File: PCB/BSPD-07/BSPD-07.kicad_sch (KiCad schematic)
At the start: 55 parts, among them IC1 LM393LVQDRQ1, IC2 LM393LVQDRQ1, IC3 LM393LVQDRQ1, IC4 LDO40LPU50RY, IC5 74LVC1G02GW-Q100H, J1 DTM13-12PA, Q1 RSQ025P03HZGTR, Q2 RJU002N06FRAT106, Q3 RJU002N06FRAT106, U2 TLP175A / COMUS AB38-Q

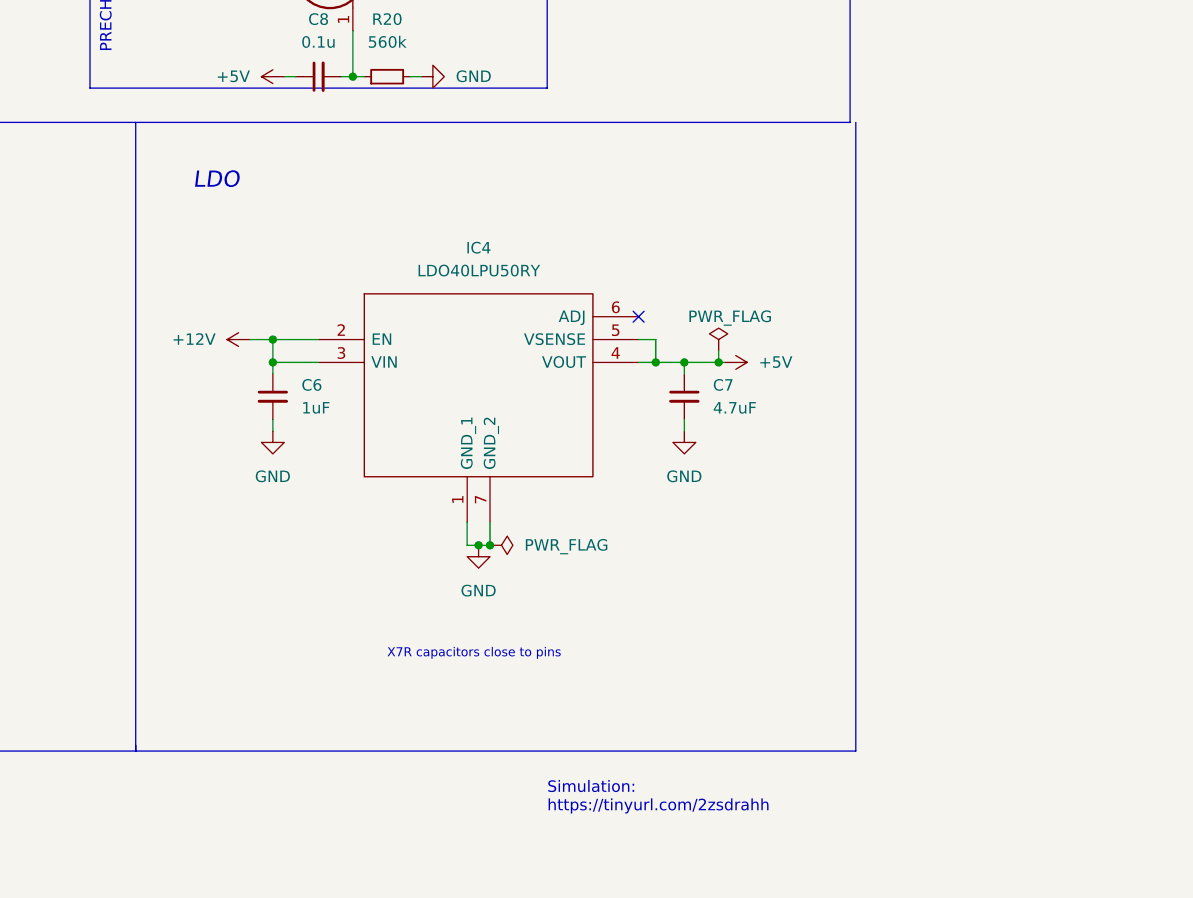
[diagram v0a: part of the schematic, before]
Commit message: Revised layout
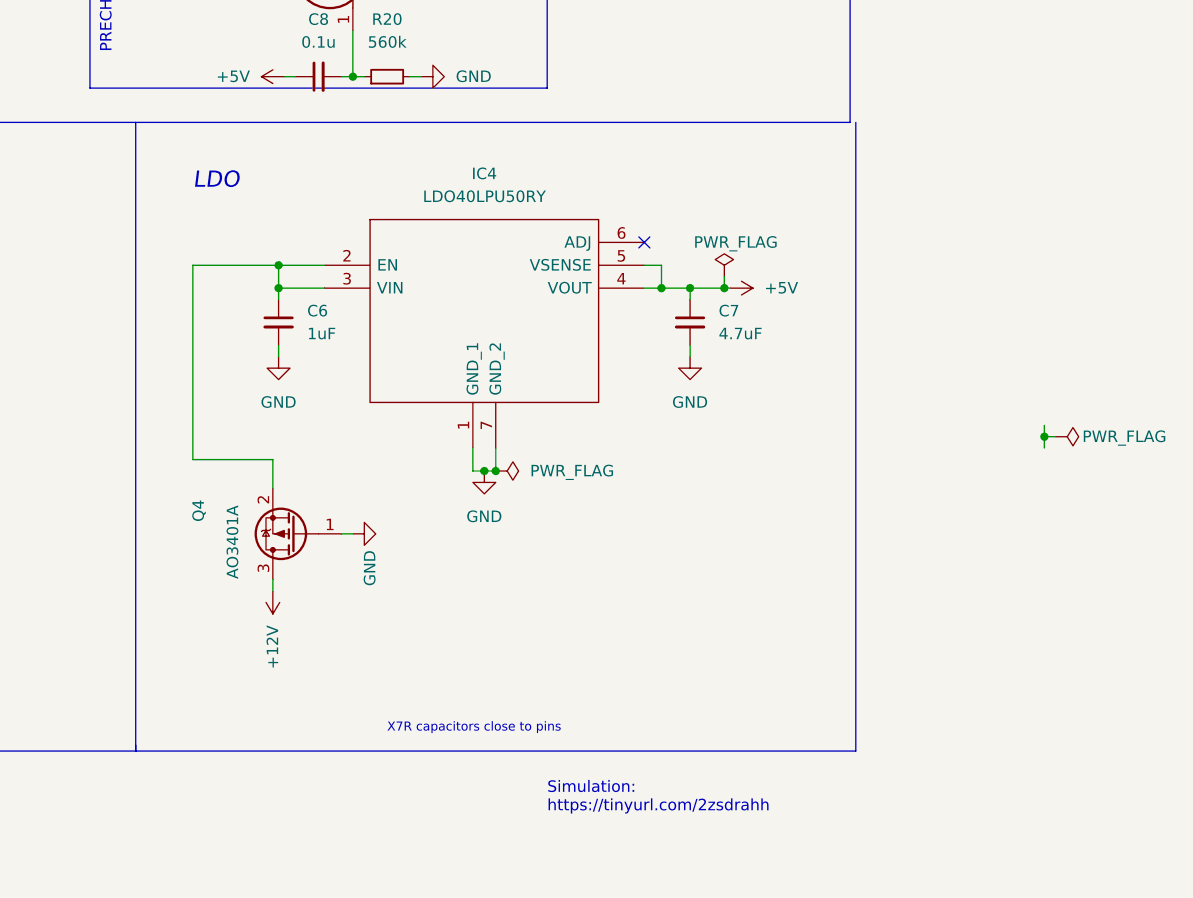
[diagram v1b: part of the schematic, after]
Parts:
- added Q4: AO3401A, Package_TO_SOT_SMD:SOT-23, symbol Transistor_FET:AO3401A
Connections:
- net +12V: now also Q4.3 (D); no longer C6.1, IC4.2 (EN), IC4.3 (VIN)
- net GND: now also Q4.1 (G)
- new net: C6.1, IC4.2 (EN), IC4.3 (VIN), Q4.2 (S)
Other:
- moved on the sheet: C6, C7, IC4
